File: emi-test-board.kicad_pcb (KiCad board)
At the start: 2 copper layers, 9 parts, among them J1 Conn_01x02_Pin, U1 XL1509-3.3

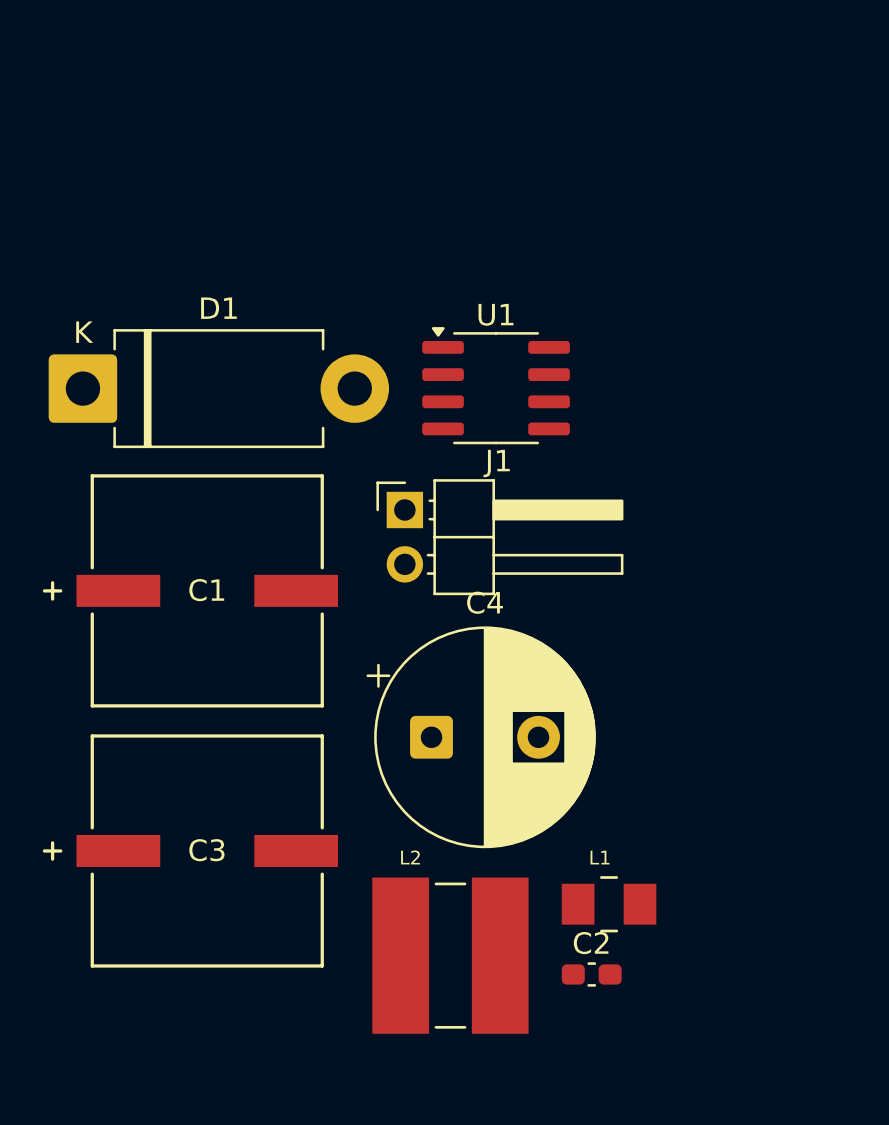
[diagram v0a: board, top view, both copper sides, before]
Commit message: feat: layout and routing
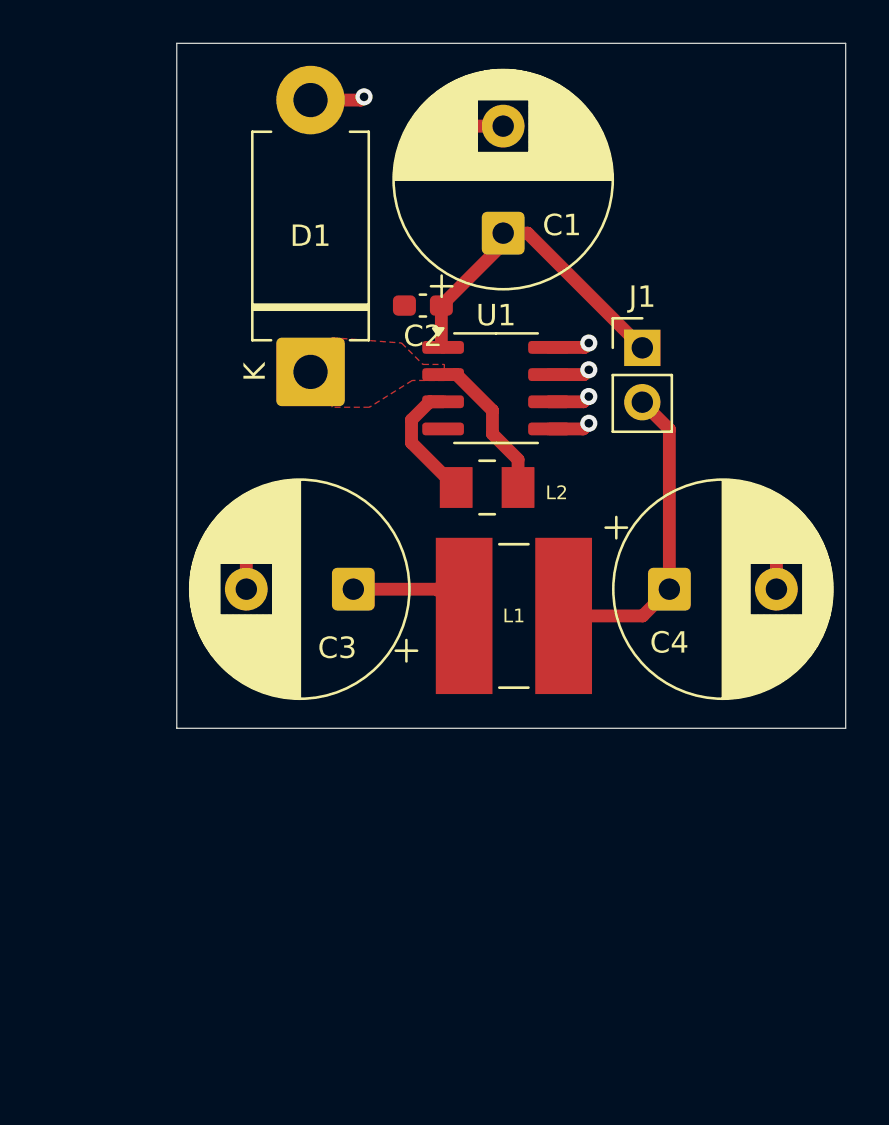
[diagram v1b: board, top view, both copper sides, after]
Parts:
- C1, C3: footprint project_footprints:PCAP_10x10-ELECT_NCA -> Capacitor_THT:CP_Radial_D10.0mm_P5.00mm
- J1: footprint Connector_PinHeader_2.54mm:PinHeader_1x02_P2.54mm_Horizontal -> Connector_PinHeader_2.54mm:PinHeader_1x02_P2.54mm_Vertical
- moved C2 32.2 mm to (96.8, 58.2), turned to 180 degrees
- moved C1 21.7 mm to (100.5, 54.9), turned to 90 degrees
- moved L1 20.3 mm to (99.8, 66.8), turned to 180 degrees
- moved L2 16.1 mm to (101.0, 72.8)
- moved C3 14.0 mm to (93.5, 71.5), turned to 180 degrees
- moved J1 13.4 mm to (107.0, 60.2)
- moved C4 13.1 mm to (108.3, 71.5)
- moved D1 10.7 mm to (91.5, 61.4), turned to 90 degrees
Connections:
- net Net-(D1-K) renamed /BUCK_OUT
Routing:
- net GND: track 0.00 -> 17.7 mm, vias 0 -> 8
- net VDD: track 0.00 -> 15.3 mm
- net +3V3 Buck: track 0.00 -> 14.7 mm
- net Net-(U1-FB): track 0.00 -> 11.5 mm
- net /BUCK_OUT: track 0.00 -> 7.09 mm
- added copper zone on F.Cu, net /BUCK_OUT
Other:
- board outline added: 31.2 x 32 mm

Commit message: rework layout
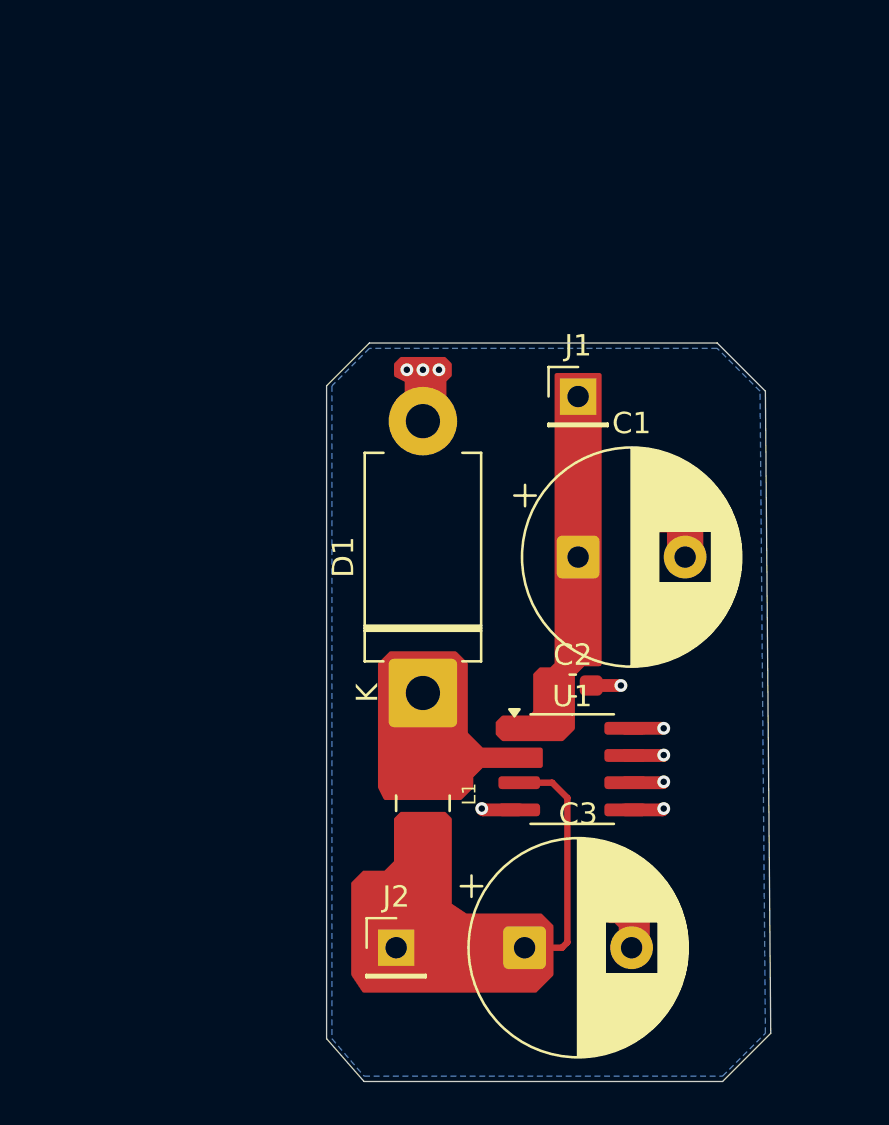
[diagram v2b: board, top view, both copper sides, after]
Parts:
- removed C4: 180uF, Capacitor_THT:CP_Radial_D10.0mm_P5.00mm
- removed L2: 3uH, project_footprints:IND_ASPI-0602S-3R0M-T
- added J2: Conn_01x02_Pin, Connector_PinHeader_2.54mm:PinHeader_1x01_P2.54mm_Vertical, F.Cu at (95.5, 88.2)
- J1: footprint Connector_PinHeader_2.54mm:PinHeader_1x02_P2.54mm_Vertical -> Connector_PinHeader_2.54mm:PinHeader_1x01_P2.54mm_Vertical
- moved C2 19.1 mm to (103.8, 76.0), turned to 0 degrees
- moved C3 18.6 mm to (101.5, 88.2), turned to 0 degrees
- moved U1 18.1 mm to (103.7, 79.9)
- moved D1 15.9 mm to (96.8, 76.3)
- moved C1 15.5 mm to (104.0, 70.0), turned to 0 degrees
- moved L1 15.1 mm to (96.8, 81.5), turned to -90 degrees
- moved J1 3.77 mm to (104.0, 62.5)
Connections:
- net /BUCK_OUT renamed /BUCK_SW
- C3 pad 1: Net-(U1-FB) -> +3V3 Buck
- L1 pad 2: Net-(U1-FB) -> +3V3 Buck
- U1 pad 3: Net-(U1-FB) -> +3V3 Buck
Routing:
- net VDD: track 15.3 -> 0.00 mm
- net Net-(U1-FB): track 11.5 -> 0.00 mm
- net GND: track 17.7 -> 10.4 mm, vias 8 -> 15
- net /BUCK_SW: track 7.09 -> 0.00 mm
- net +3V3 Buck: track 14.7 -> 11.4 mm
- added copper zone on B.Cu, net GND
- removed copper zone on F.Cu, net /BUCK_SW
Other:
- board size 31.2 x 32 mm -> 20.8 x 34.5 mm
